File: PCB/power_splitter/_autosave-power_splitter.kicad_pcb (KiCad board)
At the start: 2 copper layers, 56 x 48 mm, 34 parts, among them J1 B02P-VL, J2 B02P-VL, J3 B02P-VL, J4 PJ-082BH, J5 B02P-VL, Q2 IRLZ44N, U1 AP62300TWU, U2 AP62300TWU

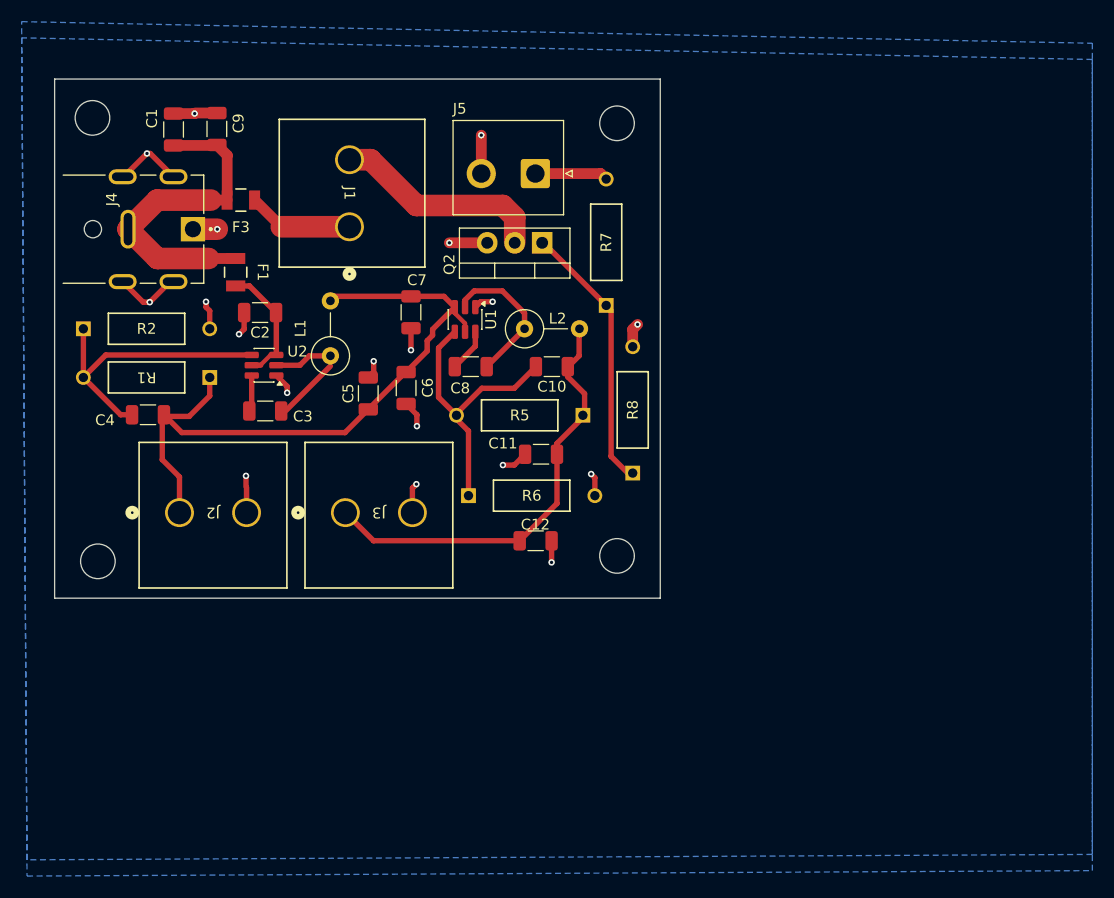
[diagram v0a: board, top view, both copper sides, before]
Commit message: Liv's stuff
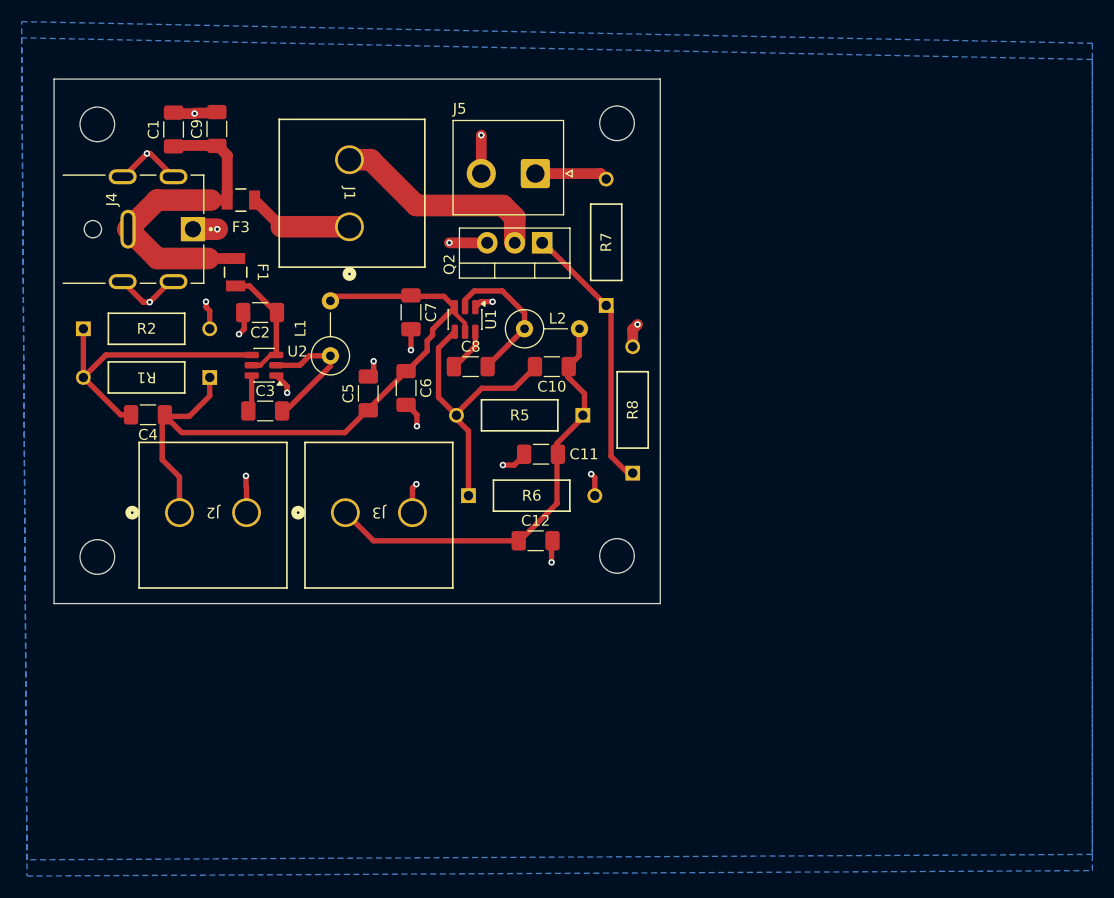
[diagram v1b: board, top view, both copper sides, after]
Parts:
- C1, C10, C11, C12, C2, C3, C4, C5, C6, C7, C8, C9: footprint Capacitor_SMD:C_1206_3216Metric -> Capacitor_SMD:C_1206_3216Metric_Pad1.33x1.80mm_HandSolder
- moved REF** 0.75 mm to (81.5, 34.5)
- moved REF** 0.40 mm to (81.5, 74.5)
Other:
- board size 56 x 48 mm -> 56.1 x 48.5 mm
